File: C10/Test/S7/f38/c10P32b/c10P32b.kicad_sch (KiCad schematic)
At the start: 5 parts

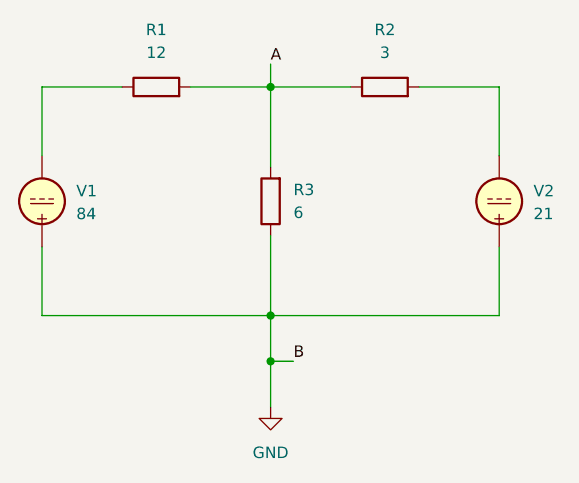
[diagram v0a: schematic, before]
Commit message: additiona upload Chapter 10
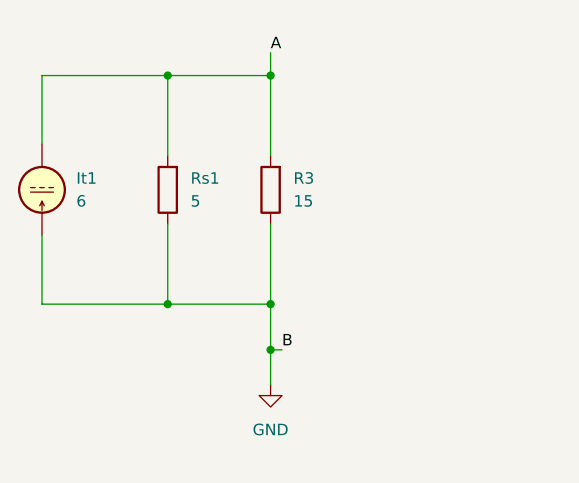
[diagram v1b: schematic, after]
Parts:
- removed R1: 12, symbol Device:R
- removed R2: 3, symbol Device:R
- removed V1: 84, symbol Simulation_SPICE:VDC
- removed V2: 21, symbol Simulation_SPICE:VDC
- added It1: 6, symbol Simulation_SPICE:IDC
- added Rs1: 5, symbol Device:R
- R3: value 6 -> 15
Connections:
- net A: now also It1.2, Rs1.2
- net GND: now also It1.1, Rs1.1
